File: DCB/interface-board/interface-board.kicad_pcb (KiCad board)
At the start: 2 copper layers, 96.5 x 76.2 mm, 13 parts, among them J1 Conn_01x14, J2 Conn_01x05, SW1 SW_SPST, SW2 SW_SPST, SW3 SW_Push_LED, SW4 SW_Push

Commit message: touching up layout and making gerbers
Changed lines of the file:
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@@
       (outputformat 1)
       (mirror false)
-      (drillshape 1)
+      (drillshape 0)
       (scaleselection 1)
-      (outputdirectory "")
+      (outputdirectory "Interface_Gerber/")
     )
   )
@@
     (fp_line (start -2.45 -3.9) (end -1.25 -3.9) (layer "F.Fab") (width 0.1))
     (fp_line (start 6.25 -3.9) (end 6.25 0.6) (layer "F.Fab") (width 0.1))
-    (pad "1" thru_hole roundrect (at 0 0 270) (size 1.7 1.95) (drill 0.95) (layers *.Cu *.Mask) (roundrect_rratio 0.147059)
+    (pad "1" thru_hole roundrect (at 0 0 270) (size 1.7 1.95) (drill 0.95) (layers *.Cu *.Mask) (roundrect_rratio 0.1470588235)
       (net 4 "+5V") (pinfunction "1") (pintype "passive"))
     (pad "2" thru_hole oval (at 2.5 0 270) (size 1.7 1.95) (drill 0.95) (layers *.Cu *.Mask)
@@
     (fp_line (start 6.25 0.6) (end 2.5 0.6) (layer "F.Fab") (width 0.1))
     (fp_line (start 2.5 7.6) (end -2.45 7.6) (layer "F.Fab") (width 0.1))
-    (pad "1" thru_hole roundrect (at 0 0 270) (size 1.7 1.95) (drill 0.95) (layers *.Cu *.Mask) (roundrect_rratio 0.147059)
+    (pad "1" thru_hole roundrect (at 0 0 270) (size 1.7 1.95) (drill 0.95) (layers *.Cu *.Mask) (roundrect_rratio 0.1470588235)
       (net 4 "+5V") (pinfunction "1") (pintype "passive"))
     (pad "2" thru_hole oval (at 2.5 0 270) (size 1.7 1.95) (drill 0.95) (layers *.Cu *.Mask)
@@
     (fp_line (start 12.45 7.6) (end 12.45 -3.9) (layer "F.Fab") (width 0.1))
     (fp_line (start -2.45 7.6) (end -2.45 -3.9) (layer "F.Fab") (width 0.1))
-    (pad "1" thru_hole roundrect (at 0 0 90) (size 1.7 1.95) (drill 0.95) (layers *.Cu *.Mask) (roundrect_rratio 0.147059)
+    (pad "1" thru_hole roundrect (at 0 0 90) (size 1.7 1.95) (drill 0.95) (layers *.Cu *.Mask) (roundrect_rratio 0.1470588235)
       (net 4 "+5V") (pinfunction "Pin_1") (pintype "passive"))
     (pad "2" thru_hole oval (at 2.5 0 90) (size 1.7 1.95) (drill 0.95) (layers *.Cu *.Mask)
@@
     (fp_line (start 3.75 7.6) (end -2.45 7.6) (layer "F.Fab") (width 0.1))
     (fp_line (start 9.95 7.6) (end 9.95 -3.9) (layer "F.Fab") (width 0.1))
-    (pad "1" thru_hole roundrect (at 0 0 90) (size 1.7 1.95) (drill 0.95) (layers *.Cu *.Mask) (roundrect_rratio 0.147059)
+    (pad "1" thru_hole roundrect (at 0 0 90) (size 1.7 1.95) (drill 0.95) (layers *.Cu *.Mask) (roundrect_rratio 0.1470588235)
       (net 5 "/START_BTN") (pinfunction "1") (pintype "passive"))
     (pad "2" thru_hole oval (at 2.5 0 90) (size 1.7 1.95) (drill 0.95) (layers *.Cu *.Mask)
@@
     (fp_line (start -2.45 -3.9) (end -1.25 -3.9) (layer "F.Fab") (width 0.1))
     (fp_line (start 4.95 7.6) (end 4.95 -3.9) (layer "F.Fab") (width 0.1))
-    (pad "1" thru_hole roundrect (at 0 0 90) (size 1.7 2) (drill 1) (layers *.Cu *.Mask) (roundrect_rratio 0.147059)
+    (pad "1" thru_hole roundrect (at 0 0 90) (size 1.7 2) (drill 1) (layers *.Cu *.Mask) (roundrect_rratio 0.1470588235)
       (net 9 "/LCD_BTN") (pinfunction "1") (pintype "passive"))
     (pad "2" thru_hole oval (at 2.5 0 90) (size 1.7 2) (drill 1) (layers *.Cu *.Mask)

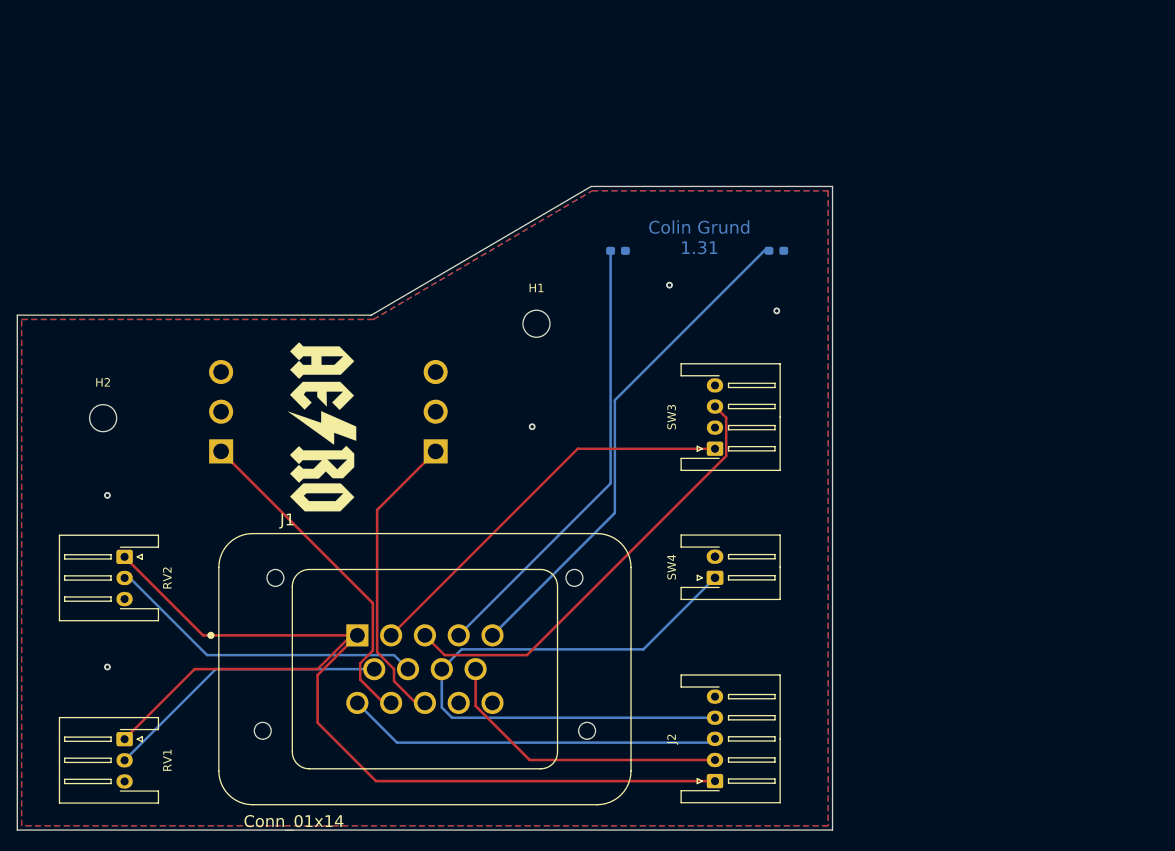
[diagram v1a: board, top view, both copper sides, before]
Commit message: Surface mount dash
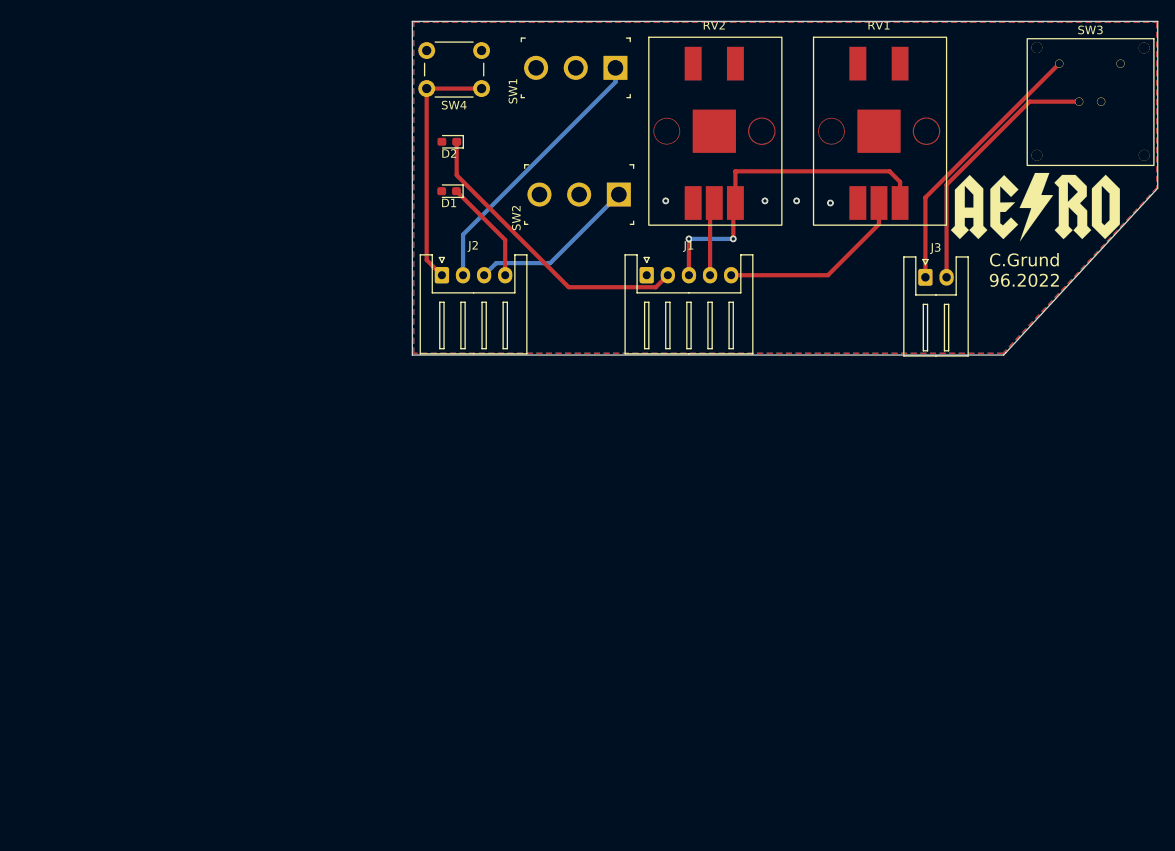
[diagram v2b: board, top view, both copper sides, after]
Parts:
- removed H1, H2: MountingHole, MountingHole:MountingHole_3.2mm_M3
- added J3: Conn_01x02, Connector_JST:JST_XH_S2B-XH-A_1x02_P2.50mm_Horizontal, F.Cu at (138.0, 76.8)
- D1, D2, SW1, SW2: moved to F.Cu
- J1: value Conn_01x14 -> Conn_01x05; footprint AERO_Footprints:TE_1-776262-1_14pin_Vertical -> Connector_JST:JST_XH_S5B-XH-A_1x05_P2.50mm_Horizontal
- J2: value Conn_01x05 -> Conn_01x04; footprint Connector_JST:JST_XH_S5B-XH-A-1_1x05_P2.50mm_Horizontal -> Connector_JST:JST_XH_S4B-XH-A_1x04_P2.50mm_Horizontal
- RV1, RV2: footprint Connector_JST:JST_XH_S3B-XH-A-1_1x03_P2.50mm_Horizontal -> AERO_Footprints:SMD_Pot
- SW3: footprint Connector_JST:JST_XH_S4B-XH-A-1_1x04_P2.50mm_Horizontal -> AERO_Footprints:LED_PUSHBUTTON
- SW4: footprint Connector_JST:JST_XH_S2B-XH-A-1_1x02_P2.50mm_Horizontal -> Button_Switch_THT:SW_PUSH_6mm
- moved RV1 114.7 mm to (132.5, 59.5), turned to 0 degrees
- moved G*** 88.4 mm to (151.0, 68.5), turned to 0 degrees
- moved RV2 86.1 mm to (113.0, 59.5), turned to 0 degrees
- moved J2 68.1 mm to (80.8, 76.5), turned to 0 degrees
- moved SW4 64.2 mm to (85.5, 54.5), turned to 180 degrees
- moved SW3 60.5 mm to (157.5, 56.0), turned to 0 degrees
- moved SW2 56.1 mm to (101.7, 67.0), turned to 180 degrees
- moved J1 53.5 mm to (105.0, 76.5)
- moved SW1 50.2 mm to (101.3, 52.0), turned to 180 degrees
- moved D2 40.8 mm to (81.6, 60.8), turned to 180 degrees
- moved D1 21.2 mm to (81.6, 66.6), turned to 180 degrees
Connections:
- J1 pad 1: +5V -> GND
- J1 pad 2: /START_BTN -> /AMS_LED
- J1 pad 3: /RTD_LED -> +5V
- J1 pad 4: /IMD_LED -> /POT_BRAKE
- J1 pad 5: /AMS_LED -> /POT_REGEN
- J2 pad 1: +5V -> /LCD_BTN
- J2 pad 2: /LCD_SCL -> /SW_DIRECTION
- J2 pad 3: /LCD_SDA -> /SW_COOLING
- J2 pad 4: /LCD_BTN -> /IMD_LED
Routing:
- net +5V: track 126.3 -> 40.2 mm, vias 0 -> 2
- net /LCD_BTN: track 74.2 -> 29.3 mm
- net /LCD_SDA: track 44.5 -> 0.00 mm
- net /IMD_LED: track 53.0 -> 12.3 mm
- net /LCD_SCL: track 35.3 -> 0.00 mm
- net /POT_BRAKE: track 38.0 -> 8.76 mm
- net /AMS_LED: track 59.4 -> 35.0 mm
- net /RTD_LED: track 52.8 -> 30.7 mm
- net /SW_COOLING: track 39.9 -> 19.9 mm
- net /START_BTN: track 47.5 -> 31.9 mm
- net /POT_REGEN: track 34.0 -> 22.5 mm
- net /SW_DIRECTION: track 35.6 -> 32.0 mm
- net GND: vias 6 -> 4
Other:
- board size 96.5 x 76.2 mm -> 88.2 x 39.5 mm
- board text added: "C.Grund 96.2022"
- board text removed: "Colin Grund 1.31"
